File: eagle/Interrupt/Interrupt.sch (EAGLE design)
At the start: 7 parts

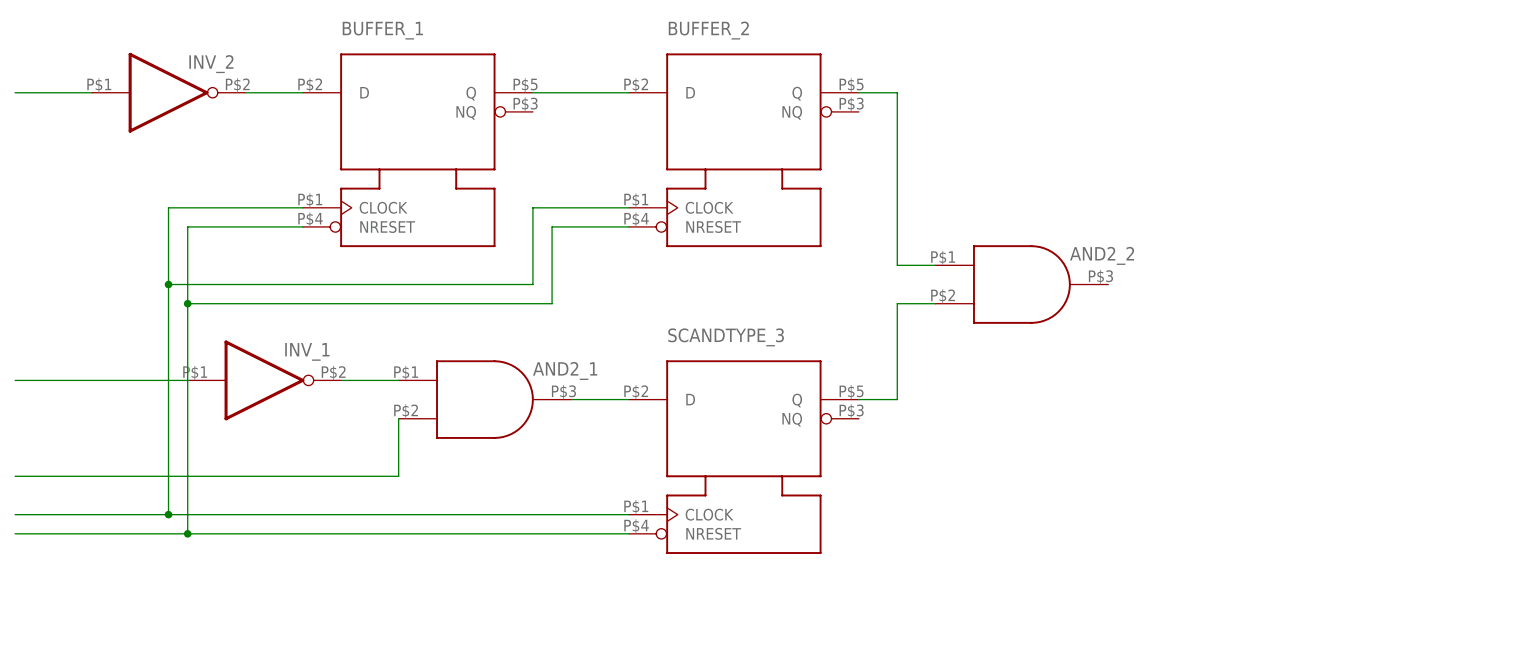
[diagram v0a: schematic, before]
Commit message: control
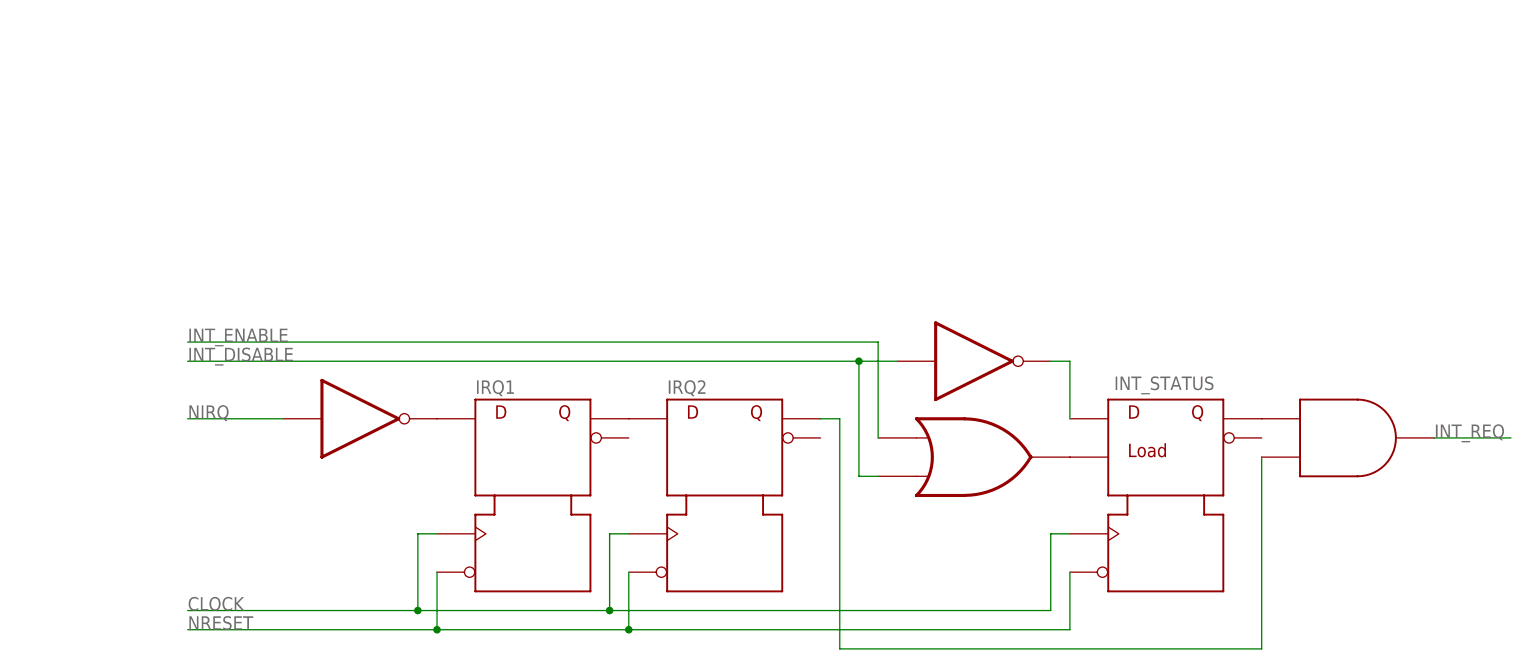
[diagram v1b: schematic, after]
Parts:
- removed AND2_2: AND2, c035u:AND2
- removed BUFFER_1, BUFFER_2, SCANDTYPE_3: SCANDTYPE, c035u:SCANDTYPE
- added INT_STATUS: SCANREG, c035u:SCANREG
- added IRQ1, IRQ2: SCANDTYPE, c035u:SCANDTYPE
- added OR2_1: OR2, c035u:OR2
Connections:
- net N$5 renamed NIRQ
- removed net N$10: BUFFER_1.NRESET, BUFFER_2.NRESET, SCANDTYPE_3.NRESET
- removed net N$11: AND2_1.A, INV_1.O
- removed net N$6: AND2_1.I1
- removed net N$8: BUFFER_1.CLOCK, BUFFER_2.CLOCK, SCANDTYPE_3.CLOCK
- removed net N$9: INV_2.I
- new net CLOCK: INT_STATUS.CLOCK, IRQ1.CLOCK, IRQ2.CLOCK
- new net INT_DISABLE: INV_2.I, OR2_1.I1
- new net INT_ENABLE: OR2_1.I0
- new net INT_REQ: AND2_1.O
- new net IRQ2: AND2_1.I1, IRQ2.Q
- new net NRESET: INT_STATUS.NRESET, IRQ1.NRESET, IRQ2.NRESET
- net N$1: now also IRQ1.Q, IRQ2.D; no longer BUFFER_1.Q, BUFFER_2.D
- net N$2: now also INV_1.O, IRQ1.D; no longer BUFFER_1.D, INV_2.O
- net N$3: now also INT_STATUS.LOAD, OR2_1.O; no longer AND2_2.A, BUFFER_2.Q
- net N$4: now also AND2_1.A, INT_STATUS.Q; no longer AND2_2.I1, SCANDTYPE_3.Q
- net N$7: now also INT_STATUS.D, INV_2.O; no longer AND2_1.O, SCANDTYPE_3.D
